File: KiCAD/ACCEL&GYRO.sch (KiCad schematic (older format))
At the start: 7 parts, among them J31 Conn_01x04, J32 Conn_01x03, J33 Conn_01x03, J34 Conn_01x04, U11 LSM6DS3

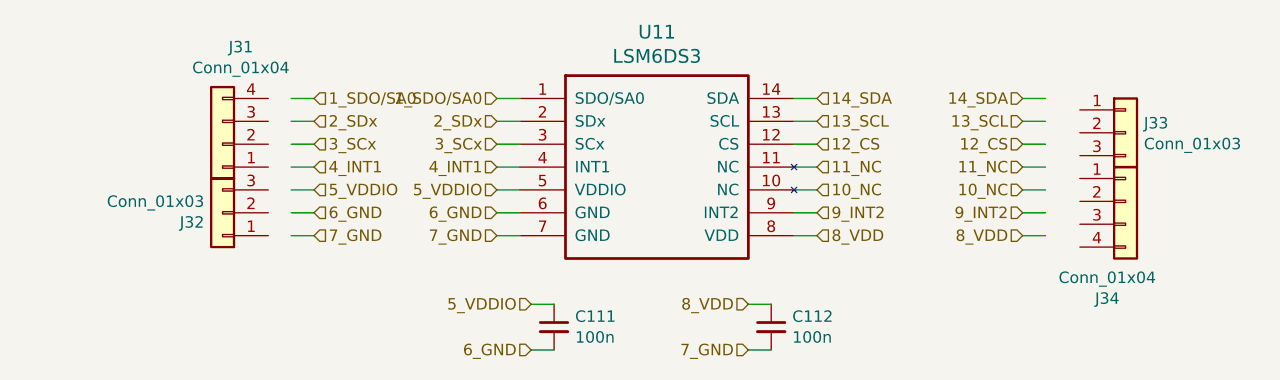
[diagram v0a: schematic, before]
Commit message: Add files via upload
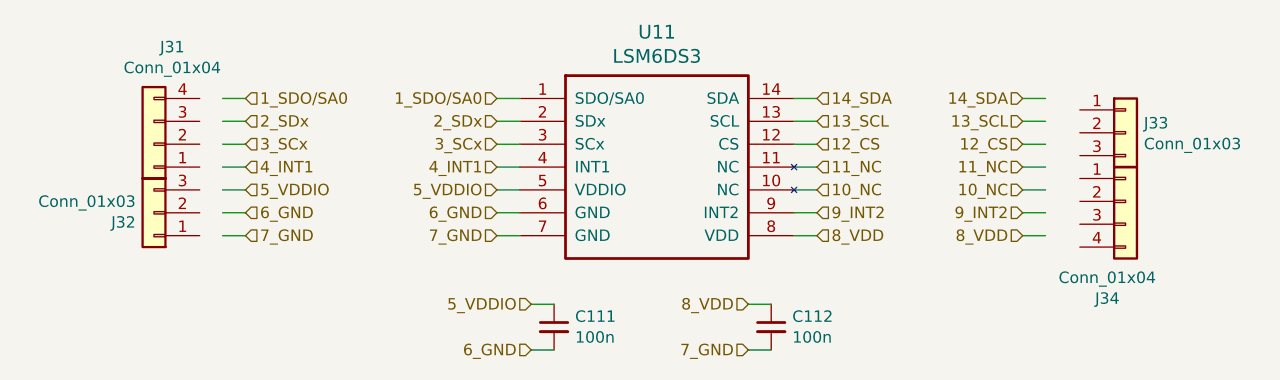
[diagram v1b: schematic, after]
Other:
- moved on the sheet: J31, J32
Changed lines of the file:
@@
 L Connector_Generic:Conn_01x03 J?
 U 1 1 5CDC27EB
-P 2500 6300
+P 2200 6300
 AR Path="/5CDC27EB" Ref="J?"  Part="1"
 AR Path="/5CDAC31F/5CDC27EB" Ref="J?"  Part="1"
@@
 AR Path="/5D23D721/5CDC27EB" Ref="J?"  Part="1"
 AR Path="/5CDC1D3D/5CDC27EB" Ref="J32"  Part="1"
-F 0 "J32" H 2580 6342 50  0000 L CNN
-F 1 "Conn_01x03" H 2580 6251 50  0000 L CNN
-F 2 "Connector_PinHeader_2.54mm:PinHeader_1x03_P2.54mm_Vertical" H 2500 6300 50  0001 C CNN
-F 3 "~" H 2500 6300 50  0001 C CNN
-	1    2500 6300
+F 0 "J32" H 2280 6342 50  0000 L CNN
+F 1 "Conn_01x03" H 2280 6251 50  0000 L CNN
+F 2 "Connector_PinHeader_2.54mm:PinHeader_1x03_P2.54mm_Vertical" H 2200 6300 50  0001 C CNN
+F 3 "~" H 2200 6300 50  0001 C CNN
+	1    2200 6300
 	-1   0    0    1
 $EndComp
@@
 L Connector_Generic:Conn_01x04 J?
 U 1 1 5CDC2CFF
-P 2500 6000
+P 2200 6000
 AR Path="/5CDC2CFF" Ref="J?"  Part="1"
 AR Path="/5CDACD1E/5CDC2CFF" Ref="J?"  Part="1"
 AR Path="/5CDC1D3D/5CDC2CFF" Ref="J31"  Part="1"
-F 0 "J31" H 2420 5575 50  0000 C CNN
-F 1 "Conn_01x04" H 2420 5666 50  0000 C CNN
-F 2 "Connector_PinHeader_2.54mm:PinHeader_1x04_P2.54mm_Vertical" H 2500 6000 50  0001 C CNN
-F 3 "~" H 2500 6000 50  0001 C CNN
-	1    2500 6000
+F 0 "J31" H 2120 5575 50  0000 C CNN
+F 1 "Conn_01x04" H 2120 5666 50  0000 C CNN
+F 2 "Connector_PinHeader_2.54mm:PinHeader_1x04_P2.54mm_Vertical" H 2200 6000 50  0001 C CNN
+F 3 "~" H 2200 6000 50  0001 C CNN
+	1    2200 6000
 	-1   0    0    1
 $EndComp
-Text HLabel 2900 6200 2    50   Input ~ 0
+Text HLabel 2600 6200 2    50   Input ~ 0
 5_VDDIO
 Wire Wire Line
-	2900 6200 2800 6200
-Text HLabel 2900 6400 2    50   Input ~ 0
+	2600 6200 2500 6200
+Text HLabel 2600 6400 2    50   Input ~ 0
 7_GND
 Wire Wire Line
-	2900 6400 2800 6400
+	2600 6400 2500 6400
 $Comp
 L Device:C_Small C?
@@
 	1    0    0    -1
 $EndComp
-Text HLabel 2900 5800 2    50   Input ~ 0
+Text HLabel 2600 5800 2    50   Input ~ 0
 1_SDO/SA0
 Wire Wire Line
-	2900 5800 2800 5800
-Text HLabel 2900 6300 2    50   Input ~ 0
+	2600 5800 2500 5800
+Text HLabel 2600 6300 2    50   Input ~ 0
 6_GND
 Wire Wire Line
-	2900 6300 2800 6300
+	2600 6300 2500 6300
 $Comp
 L Device:C_Small C?
@@
 	1    0    0    -1
 $EndComp
-Text HLabel 2900 5900 2    50   Input ~ 0
+Text HLabel 2600 5900 2    50   Input ~ 0
 2_SDx
 Wire Wire Line
-	2900 5900 2800 5900
-Text HLabel 2900 6100 2    50   Input ~ 0
+	2600 5900 2500 5900
+Text HLabel 2600 6100 2    50   Input ~ 0
 4_INT1
 Wire Wire Line
-	2900 6100 2800 6100
-Text HLabel 2900 6000 2    50   Input ~ 0
+	2600 6100 2500 6100
+Text HLabel 2600 6000 2    50   Input ~ 0
 3_SCx
 Wire Wire Line
-	2900 6000 2800 6000
+	2600 6000 2500 6000
 $Comp
 L Connector_Generic:Conn_01x03 J?
